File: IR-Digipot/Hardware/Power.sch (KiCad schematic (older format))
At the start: 40 parts, among them Q7 STL6P3LLH6, U8 L7985TR, U9 LM27761

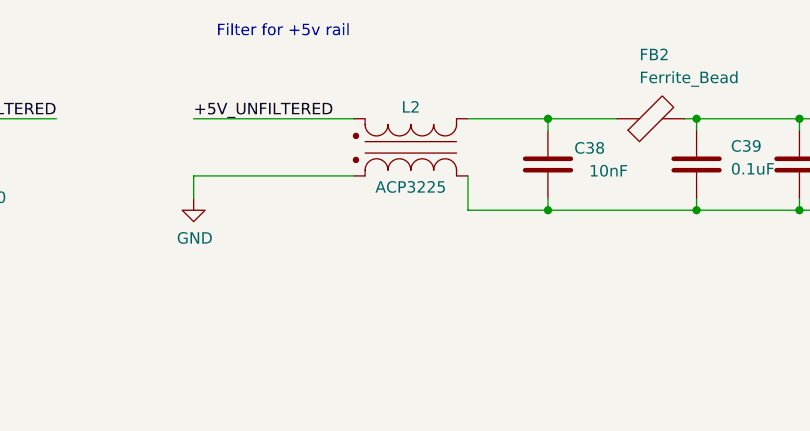
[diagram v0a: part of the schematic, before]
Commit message: Fully routed USB-C PD and +5VD regulators
Zones will need some tweaks, but electrically those circuits
are usable now.
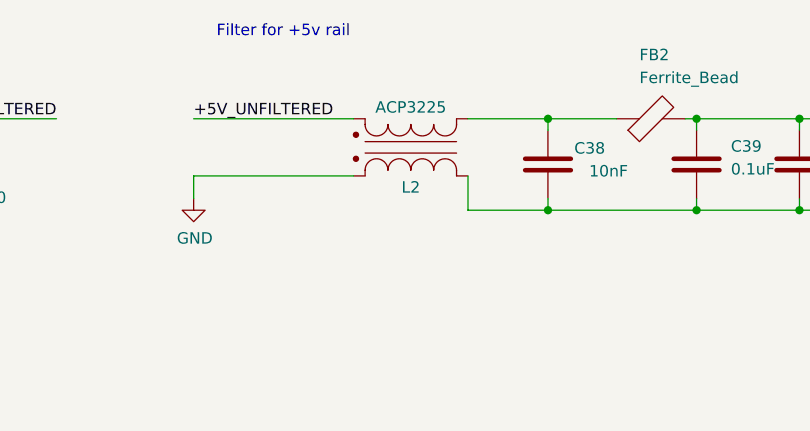
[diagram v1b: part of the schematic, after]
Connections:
- net +5V_UNFILTERED: now also L2.1; no longer L2.3
- net GND: now also L2.3; no longer L2.1
- net GNDD: now also L2.4; no longer L2.2
- net at C38.2, FB2.1: now also L2.2; no longer L2.4
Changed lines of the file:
@@
 L Library:EMI_Filter_CommonMode L2
 U 1 1 5FE9F1B9
-P 8150 1700
-F 0 "L2" H 8150 1400 50  0000 C CNN
-F 1 "ACP3225" H 8150 1750 50  0000 C CNN
-F 2 "Librray:ACP3225" H 8150 1675 50  0001 C CNN
-F 3 "0.39370078740157477" H 8150 1675 50  0001 C CNN
-F 4 "CMC 1.5A 2LN 1 KOHM SMD" H 8150 1700 50  0001 C CNN "Description"
-F 5 "TDK Corporation" H 8150 1700 50  0001 C CNN "Manufacturer"
-F 6 "ACP3225-102-2P-T000" H 8150 1700 50  0001 C CNN "Manufacturer Part Number"
-F 7 "445-8637-1-ND" H 8150 1700 50  0001 C CNN "Digi-Key Part Number"
-	1    8150 1700
-	1    0    0    1
+P 8150 1450
+F 0 "L2" H 8150 1150 50  0000 C CNN
+F 1 "ACP3225" H 8150 1500 50  0000 C CNN
+F 2 "Librray:ACP3225" H 8150 1425 50  0001 C CNN
+F 3 "0.39370078740157477" H 8150 1425 50  0001 C CNN
+F 4 "CMC 1.5A 2LN 1 KOHM SMD" H 8150 1450 50  0001 C CNN "Description"
+F 5 "TDK Corporation" H 8150 1450 50  0001 C CNN "Manufacturer"
+F 6 "ACP3225-102-2P-T000" H 8150 1450 50  0001 C CNN "Manufacturer Part Number"
+F 7 "445-8637-1-ND" H 8150 1450 50  0001 C CNN "Digi-Key Part Number"
+	1    8150 1450
+	1    0    0    -1
 $EndComp
 Wire Wire Line

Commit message: Rework power supply ground zones
USB-C PD and +5VD regulator can now be considered final: small tweaks
are possible, but overall seems all fine.
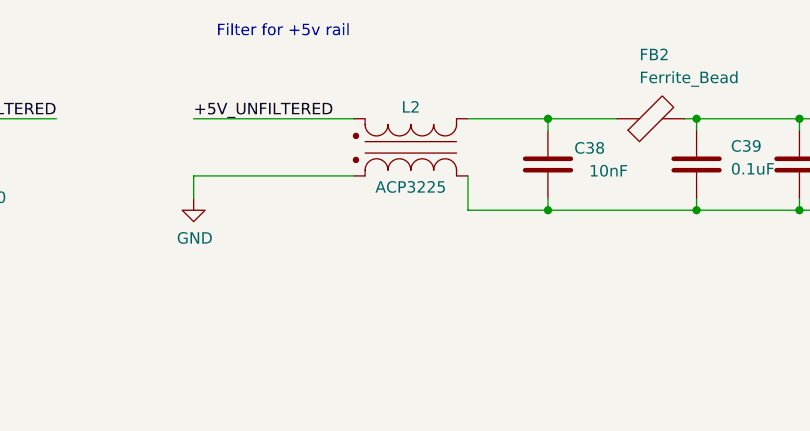
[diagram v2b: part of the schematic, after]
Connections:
- net +5V_UNFILTERED: now also L2.3; no longer L2.1
- net GND: now also L2.1; no longer L2.3
- net GNDD: now also L2.2; no longer L2.4
- net at C38.2, FB2.1: now also L2.4; no longer L2.2
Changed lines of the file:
@@
 L Library:EMI_Filter_CommonMode L2
 U 1 1 5FE9F1B9
-P 8150 1450
-F 0 "L2" H 8150 1150 50  0000 C CNN
-F 1 "ACP3225" H 8150 1500 50  0000 C CNN
-F 2 "Librray:ACP3225" H 8150 1425 50  0001 C CNN
-F 3 "0.39370078740157477" H 8150 1425 50  0001 C CNN
-F 4 "CMC 1.5A 2LN 1 KOHM SMD" H 8150 1450 50  0001 C CNN "Description"
-F 5 "TDK Corporation" H 8150 1450 50  0001 C CNN "Manufacturer"
-F 6 "ACP3225-102-2P-T000" H 8150 1450 50  0001 C CNN "Manufacturer Part Number"
-F 7 "445-8637-1-ND" H 8150 1450 50  0001 C CNN "Digi-Key Part Number"
-	1    8150 1450
-	1    0    0    -1
+P 8150 1700
+F 0 "L2" H 8150 1400 50  0000 C CNN
+F 1 "ACP3225" H 8150 1750 50  0000 C CNN
+F 2 "Librray:ACP3225" H 8150 1675 50  0001 C CNN
+F 3 "0.39370078740157477" H 8150 1675 50  0001 C CNN
+F 4 "CMC 1.5A 2LN 1 KOHM SMD" H 8150 1700 50  0001 C CNN "Description"
+F 5 "TDK Corporation" H 8150 1700 50  0001 C CNN "Manufacturer"
+F 6 "ACP3225-102-2P-T000" H 8150 1700 50  0001 C CNN "Manufacturer Part Number"
+F 7 "445-8637-1-ND" H 8150 1700 50  0001 C CNN "Digi-Key Part Number"
+	1    8150 1700
+	1    0    0    1
 $EndComp
 Wire Wire Line
